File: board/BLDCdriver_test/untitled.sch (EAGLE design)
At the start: 28 parts, among them M1 JST-XH-03-PIN-LONG-PAD, X1 JST-XH-02-PIN-LONG-PAD, X2 JST-XH-06-PIN-ROUND-PAD, X4 JST-XH-04-PIN-ROUND-PAD

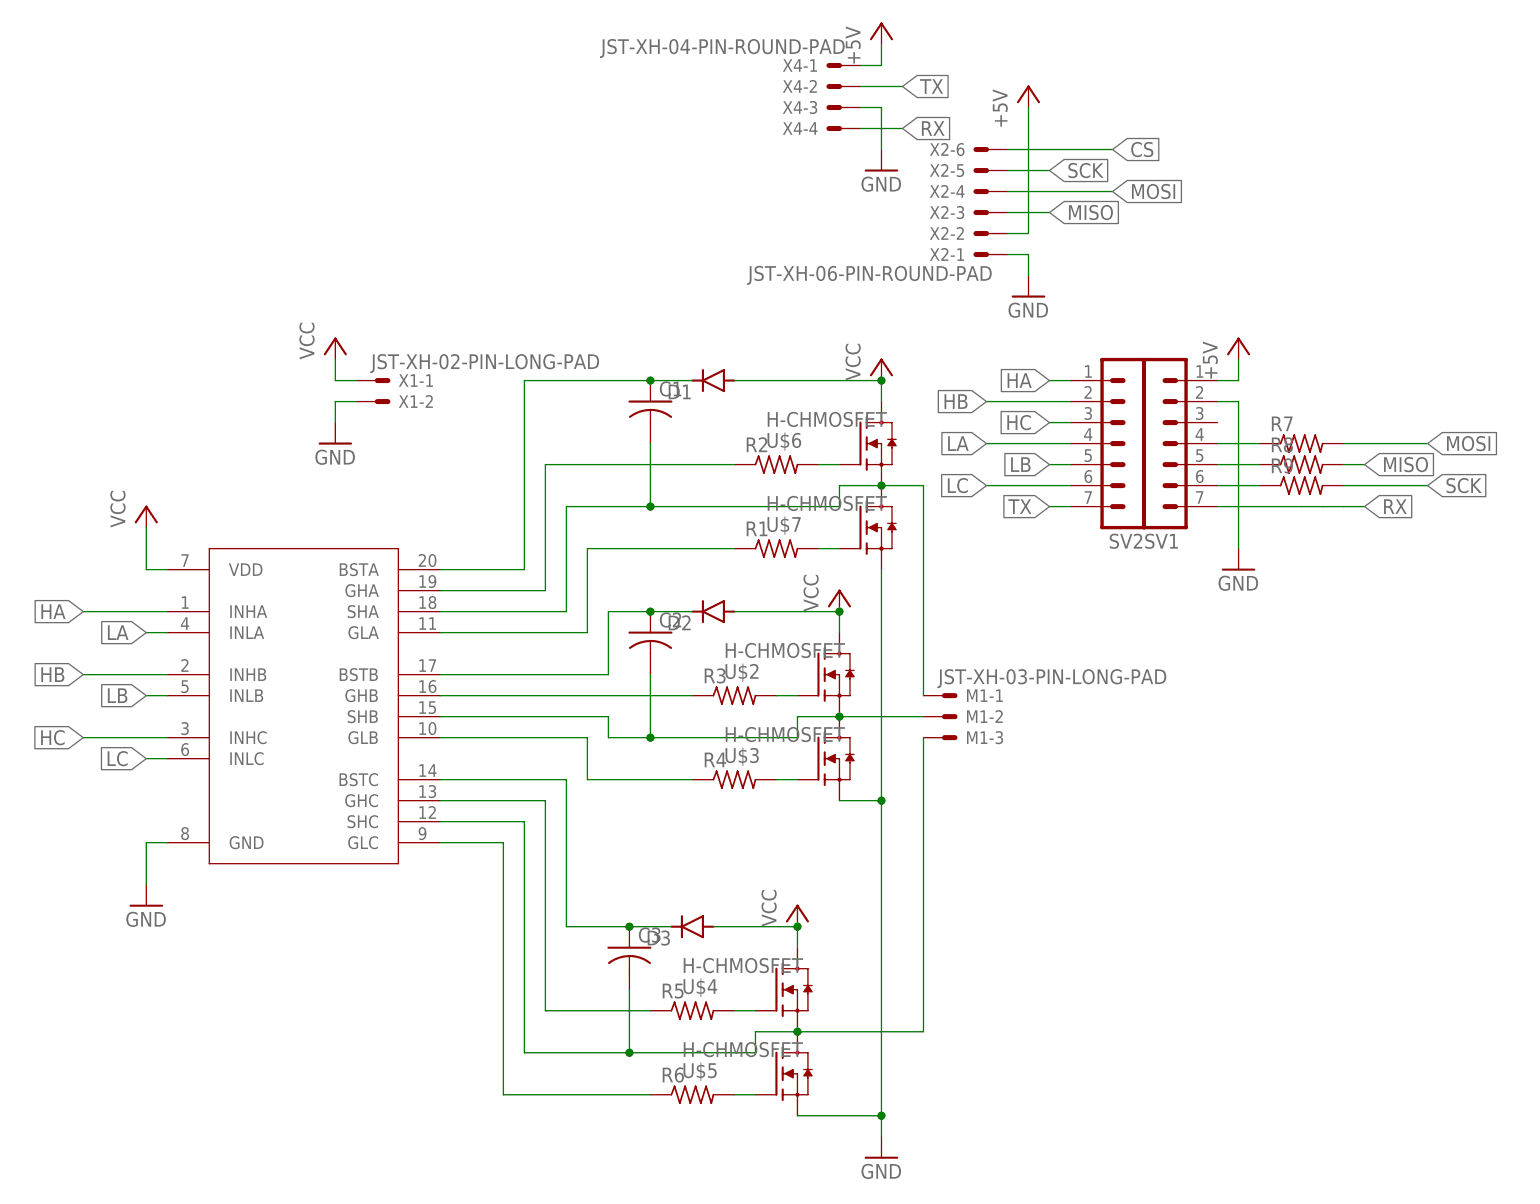
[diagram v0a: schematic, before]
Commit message: update boards 2022-07-14
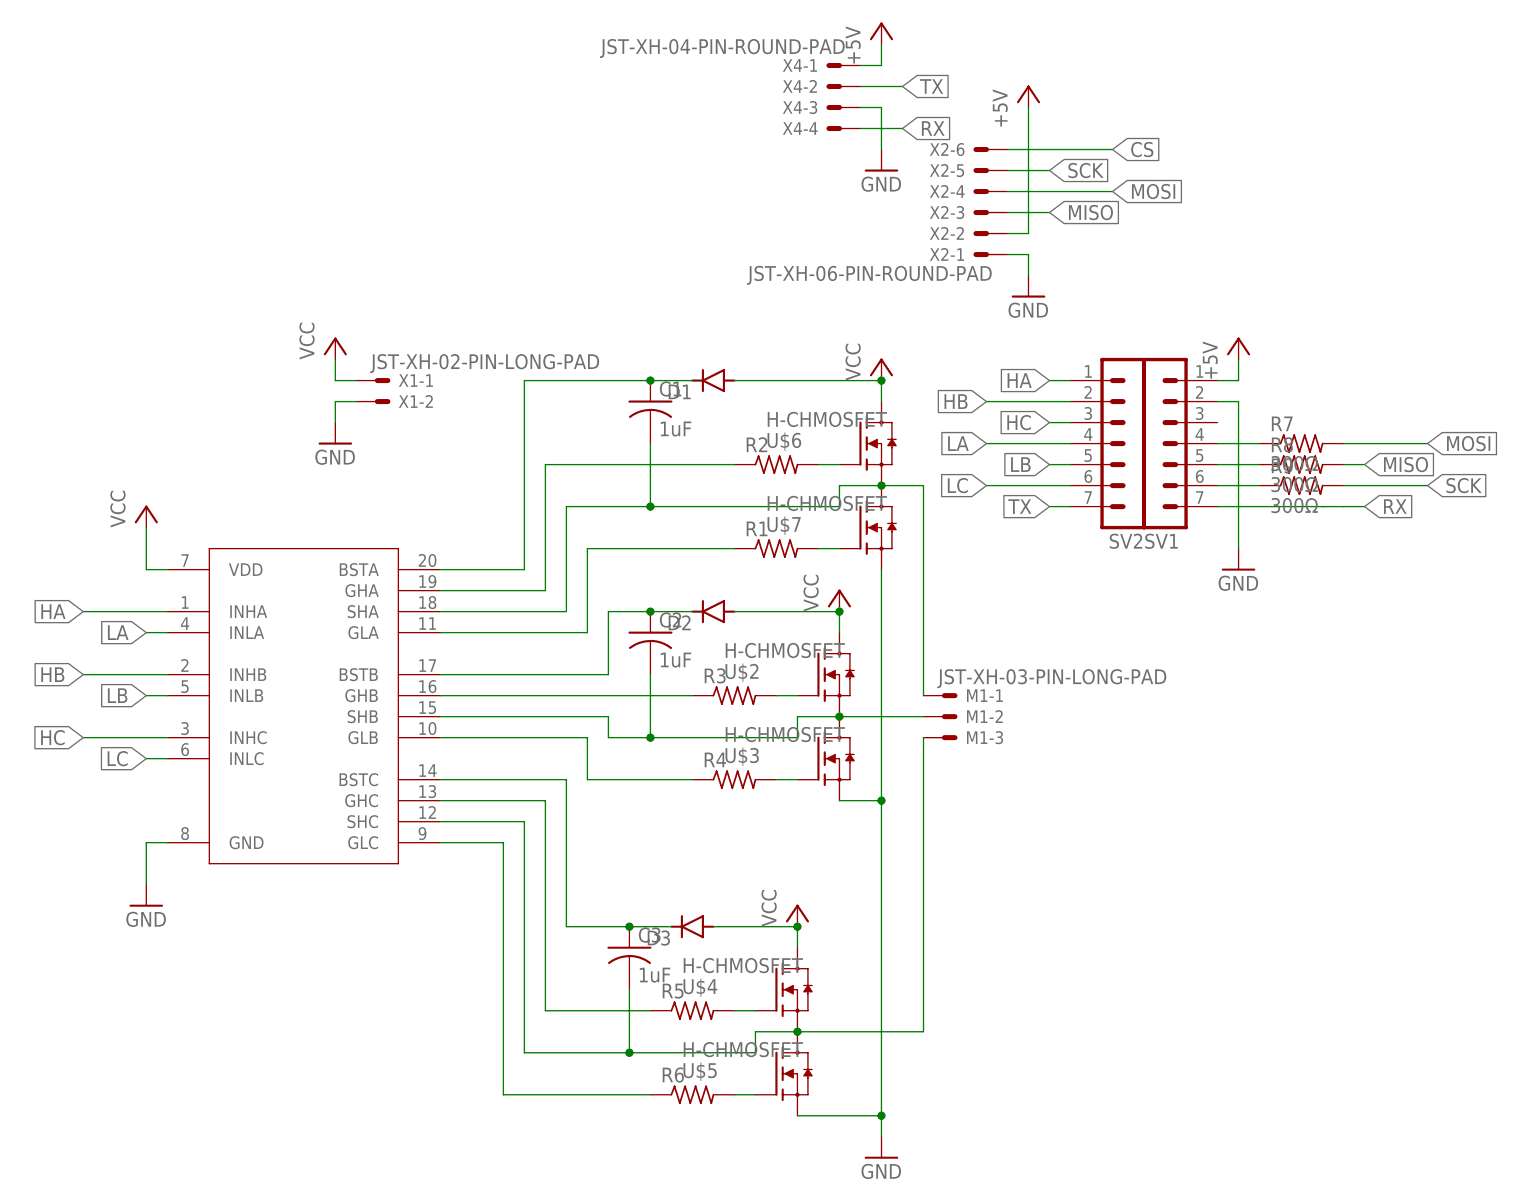
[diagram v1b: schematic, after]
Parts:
- C1, C2, C3: value (none) -> 1uF
- R7, R8, R9: value (none) -> 300Ω
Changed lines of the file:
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@@
 <part name="R3" library="adafruit" deviceset="R-US_" device="M2012"/>
 <part name="R4" library="adafruit" deviceset="R-US_" device="M2012"/>
-<part name="C1" library="adafruit" deviceset="C-US" device="C2012"/>
-<part name="C2" library="adafruit" deviceset="C-US" device="C2012"/>
+<part name="C1" library="adafruit" deviceset="C-US" device="C2012" value="1uF"/>
+<part name="C2" library="adafruit" deviceset="C-US" device="C2012" value="1uF"/>
 <part name="P+1" library="supply1" deviceset="VCC" device=""/>
 <part name="P+2" library="supply1" deviceset="VCC" device=""/>
@@
 <part name="R5" library="adafruit" deviceset="R-US_" device="M2012"/>
 <part name="R6" library="adafruit" deviceset="R-US_" device="M2012"/>
-<part name="C3" library="adafruit" deviceset="C-US" device="C2012"/>
+<part name="C3" library="adafruit" deviceset="C-US" device="C2012" value="1uF"/>
 <part name="D1" library="diode" library_urn="urn:adsk.eagle:library:210" deviceset="DIODE-" device="DO-214AC" package3d_urn="urn:adsk.eagle:package:43416/2"/>
 <part name="D2" library="diode" library_urn="urn:adsk.eagle:library:210" deviceset="DIODE-" device="DO-214AC" package3d_urn="urn:adsk.eagle:package:43416/2"/>
@@
 <part name="P+8" library="supply1" library_urn="urn:adsk.eagle:library:371" deviceset="+5V" device=""/>
 <part name="GND6" library="supply1" library_urn="urn:adsk.eagle:library:371" deviceset="GND" device=""/>
-<part name="R7" library="adafruit" deviceset="R-US_" device="M2012"/>
-<part name="R8" library="adafruit" deviceset="R-US_" device="M2012"/>
-<part name="R9" library="adafruit" deviceset="R-US_" device="M2012"/>
+<part name="R7" library="adafruit" deviceset="R-US_" device="M2012" value="300Ω"/>
+<part name="R8" library="adafruit" deviceset="R-US_" device="M2012" value="300Ω"/>
+<part name="R9" library="adafruit" deviceset="R-US_" device="M2012" value="300Ω"/>
 </parts>
 <sheets>
